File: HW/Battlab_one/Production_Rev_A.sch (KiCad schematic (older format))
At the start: 53 parts, among them IC2 MIC5225-5.0YM5-TR, J1 BANANA_CONN, J3 BANANA_CONN, P1 USB_C_Plug, T1 750315371

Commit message: manf#
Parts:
- AD5248: manf# (none) -> 584-AD5248BRMZ100
- AP2318: manf# (none) -> 621-AP2318M-ADJTRG1
- FTDI232RL1: manf# (none) -> C8690
- IC2: manf# (none) -> C145704
- INA233: manf# (none) -> 595-INA233AIDGST
- ISO1540: manf# (none) -> C179739
- ISO7742: manf# (none) -> 595-ISO7742DBQ
- MSP430: manf# (none) -> C107631
- SN6505: manf# (none) -> C74518
- T1: manf# (none) -> 710-750315371
- USBPROT1: manf# (none) -> 595-TPD2E2U06DRLR
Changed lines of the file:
@@
 	5400 8100 5800 8100
-Wire Wire Line
-	5800 8100 5800 8900
-Wire Wire Line
-	5800 8900 3800 8900
 Wire Wire Line
 	3800 8900 3800 8100
@@
 F 2 "Production_Rev_A:SSOP28DB" H 4900 5100 50  0001 C CNN
 F 3 "" H 4900 5100 50  0001 C CNN
+F 4 "C8690" H 4900 5100 50  0001 C CNN "manf#"
 	1    4900 5100
 	1    0    0    -1
@@
 F 2 "Production_Rev_A:SOIC-8" H 11000 3000 50  0001 C CNN
 F 3 "" H 11000 3000 50  0001 C CNN
+F 4 "621-AP2318M-ADJTRG1" H 11000 3000 50  0001 C CNN "manf#"
 	1    11000 3000
 	1    0    0    -1
@@
 F 2 "Production_Rev_A:VSSOP-10" H 11100 7300 50  0001 C CNN
 F 3 "" H 11100 7300 50  0001 C CNN
+F 4 "595-INA233AIDGST" H 11100 7300 50  0001 C CNN "manf#"
 	1    11100 7300
 	1    0    0    -1
@@
 F 2 "Production_Rev_A:MSOP-10" H 11000 5200 50  0001 C CNN
 F 3 "" H 11000 5200 50  0001 C CNN
+F 4 "584-AD5248BRMZ100" H 11000 5200 50  0001 C CNN "manf#"
 	1    11000 5200
 	1    0    0    -1
@@
 F 2 "Production_Rev_A:PW20" H 5000 2300 50  0001 C CNN
 F 3 "" H 5000 2300 50  0001 C CNN
+F 4 "C107631" H 5000 2300 50  0001 C CNN "manf#"
 	1    5000 2300
 	1    0    0    -1
@@
 F 2 "Production_Rev_A:TOR-6P-HT4_SMT_6PIN_(1201)" H 7900 7400 50  0001 C CNN
 F 3 "" H 7900 7400 50  0001 C CNN
+F 4 "710-750315371" H 7900 7400 50  0001 C CNN "manf#"
 	1    7900 7400
-	1    0    0    -1
-$EndComp
-$Comp
-L Production_Rev_A-eagle-import:SN6505 SN6505
-U 1 1 5779FEE2
-P 5400 8500
-F 0 "SN6505" H 4700 9500 42  0000 L BNN
-F 1 "SN6505" H 4700 8200 42  0000 L BNN
-F 2 "Production_Rev_A:SOT95P280X145-6N" H 5400 8500 50  0001 C CNN
-F 3 "" H 5400 8500 50  0001 C CNN
-	1    5400 8500
 	1    0    0    -1
 $EndComp
@@
 F 2 "Production_Rev_A:SOIC127P600X175-8N" H 9100 5600 50  0001 C CNN
 F 3 "" H 9100 5600 50  0001 C CNN
+F 4 "C179739" H 9100 5600 50  0001 C CNN "manf#"
 	1    9100 5600
 	1    0    0    -1
@@
 F 2 "Production_Rev_A:SOP63P599X175-16N" H 7900 2100 50  0001 C CNN
 F 3 "" H 7900 2100 50  0001 C CNN
+F 4 "595-ISO7742DBQ" H 7900 2100 50  0001 C CNN "manf#"
 	1    7900 2100
 	1    0    0    -1
@@
 F 2 "Production_Rev_A:SOT50P160X60-5N" H 2000 6300 50  0001 C CNN
 F 3 "" H 2000 6300 50  0001 C CNN
+F 4 "595-TPD2E2U06DRLR" H 2000 6300 50  0001 C CNN "manf#"
 	1    2000 6300
 	-1   0    0    1
@@
 F 2 "Production_Rev_A:SOT95P280X130-5N" H 10400 8700 50  0001 C CNN
 F 3 "" H 10400 8700 50  0001 C CNN
+F 4 "C145704" H 10400 8700 50  0001 C CNN "manf#"
 	1    10400 8700
 	1    0    0    -1
@@
 	1505 2165 1650 2165
 Connection ~ 1650 2165
+Wire Wire Line
+	5800 8900 3800 8900
+Wire Wire Line
+	5800 8100 5800 8900
+$Comp
+L Production_Rev_A-eagle-import:SN6505 SN6505
+U 1 1 5779FEE2
+P 5400 8500
+F 0 "SN6505" H 4700 9500 42  0000 L BNN
+F 1 "SN6505" H 4700 8200 42  0000 L BNN
+F 2 "Production_Rev_A:SOT95P280X145-6N" H 5400 8500 50  0001 C CNN
+F 3 "" H 5400 8500 50  0001 C CNN
+F 4 "C74518" H 5400 8500 50  0001 C CNN "manf#"
+	1    5400 8500
+	1    0    0    -1
+$EndComp
 $EndSCHEMATC

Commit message: manf#
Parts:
- C1, C10, C4: manf# (none) -> C123655
- C11, C14, C16, C17, C5, C7, C8: manf# (none) -> C110253
- C12, C13: manf# (none) -> C513774
- C15, C2, C6: manf# (none) -> C141195
- C3: manf# (none) -> C249843
- C9: manf# (none) -> C1845
- D2, D3: manf# (none) -> 863-MBR0520LT1G
- D4: manf# (none) -> C375460
- J1, J3: manf# (none) -> C106273
- P-MOS1: manf# (none) -> C518789
- P1: manf# (none) -> C393939
- R1, R2, R6, R7: manf# (none) -> C104602
- R10, R9: manf# (none) -> C164004
- R11, R12: manf# (none) -> C137353
- R13: manf# (none) -> C702843
- R14, R8: manf# (none) -> C723762
- R15: manf# (none) -> C149672
- R3: manf# (none) -> C104814
- R4, R5: manf# (none) -> C429214
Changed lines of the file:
@@
 F 2 "Production_Rev_A:1206" H 6800 4100 50  0001 C CNN
 F 3 "" H 6800 4100 50  0001 C CNN
+F 4 "C104602" H 6800 4100 50  0001 C CNN "manf#"
 	1    6800 4100
 	0    -1   -1   0
@@
 F 2 "Production_Rev_A:1206" H 7000 4100 50  0001 C CNN
 F 3 "" H 7000 4100 50  0001 C CNN
+F 4 "C104602" H 7000 4100 50  0001 C CNN "manf#"
 	1    7000 4100
 	0    -1   -1   0
@@
 F 2 "Production_Rev_A:1206" H 12300 5400 50  0001 C CNN
 F 3 "" H 12300 5400 50  0001 C CNN
+F 4 "C141195" H 12300 5400 50  0001 C CNN "manf#"
 	1    12300 5400
 	1    0    0    -1
@@
 F 2 "Production_Rev_A:1206" H 14600 3300 50  0001 C CNN
 F 3 "" H 14600 3300 50  0001 C CNN
+F 4 "C149672" H 14600 3300 50  0001 C CNN "manf#"
 	1    14600 3300
 	1    0    0    -1
@@
 F 2 "Production_Rev_A:1206" H 10300 3600 50  0001 C CNN
 F 3 "" H 10300 3600 50  0001 C CNN
+F 4 "C123655" H 10300 3600 50  0001 C CNN "manf#"
 	1    10300 3600
 	-1   0    0    1
@@
 F 2 "Production_Rev_A:PANASONIC_F" H 15700 3000 50  0001 C CNN
 F 3 "" H 15700 3000 50  0001 C CNN
+F 4 "C249843" H 15700 3000 50  0001 C CNN "manf#"
 	1    15700 3000
 	-1   0    0    1
@@
 F 2 "Production_Rev_A:1206" H 4100 3100 50  0001 C CNN
 F 3 "" H 4100 3100 50  0001 C CNN
+F 4 "C110253" H 4100 3100 50  0001 C CNN "manf#"
 	1    4100 3100
 	0    1    1    0
@@
 F 2 "Production_Rev_A:1206" H 4800 1200 50  0001 C CNN
 F 3 "" H 4800 1200 50  0001 C CNN
+F 4 "C429214" H 4800 1200 50  0001 C CNN "manf#"
 	1    4800 1200
 	1    0    0    -1
@@
 F 2 "Production_Rev_A:1206" H 6400 2300 50  0001 C CNN
 F 3 "" H 6400 2300 50  0001 C CNN
+F 4 "C1845" H 6400 2300 50  0001 C CNN "manf#"
 	1    6400 2300
 	0    1    1    0
@@
 F 2 "Production_Rev_A:1206" H 3100 3100 50  0001 C CNN
 F 3 "" H 3100 3100 50  0001 C CNN
+F 4 "C429214" H 3100 3100 50  0001 C CNN "manf#"
 	1    3100 3100
 	-1   0    0    1
@@
 F 2 "Production_Rev_A:1206" H 6500 1400 50  0001 C CNN
 F 3 "" H 6500 1400 50  0001 C CNN
+F 4 "C137353" H 6500 1400 50  0001 C CNN "manf#"
 	1    6500 1400
 	1    0    0    -1
@@
 F 2 "Production_Rev_A:1206" H 16000 3010 50  0001 C CNN
 F 3 "" H 16000 3010 50  0001 C CNN
+F 4 "C110253" H 16000 3010 50  0001 C CNN "manf#"
 	1    16000 3010
 	1    0    0    -1
@@
 F 2 "Production_Rev_A:1206" H 3800 9300 50  0001 C CNN
 F 3 "" H 3800 9300 50  0001 C CNN
+F 4 "C513774" H 3800 9300 50  0001 C CNN "manf#"
 	1    3800 9300
 	1    0    0    -1
@@
 F 2 "Production_Rev_A:SOD3716X117(SOD-123)" H 8800 7100 50  0001 C CNN
 F 3 "" H 8800 7100 50  0001 C CNN
+F 4 "863-MBR0520LT1G" H 8800 7100 50  0001 C CNN "manf#"
 	1    8800 7100
 	1    0    0    -1
@@
 F 2 "Production_Rev_A:SOD3716X117(SOD-123)" H 8900 7700 50  0001 C CNN
 F 3 "" H 8900 7700 50  0001 C CNN
+F 4 "863-MBR0520LT1G" H 8900 7700 50  0001 C CNN "manf#"
 	1    8900 7700
 	1    0    0    -1
@@
 F 2 "Production_Rev_A:1206" H 9300 8100 50  0001 C CNN
 F 3 "" H 9300 8100 50  0001 C CNN
+F 4 "C513774" H 9300 8100 50  0001 C CNN "manf#"
 	1    9300 8100
 	1    0    0    -1
@@
 F 2 "Production_Rev_A:1206" H 9800 8100 50  0001 C CNN
 F 3 "" H 9800 8100 50  0001 C CNN
+F 4 "C110253" H 9800 8100 50  0001 C CNN "manf#"
 	1    9800 8100
 	1    0    0    -1
@@
 F 2 "Production_Rev_A:1206" H 8800 4600 50  0001 C CNN
 F 3 "" H 8800 4600 50  0001 C CNN
+F 4 "C104602" H 8800 4600 50  0001 C CNN "manf#"
 	1    8800 4600
 	0    1    1    0
@@
 F 2 "Production_Rev_A:1206" H 9100 4600 50  0001 C CNN
 F 3 "" H 9100 4600 50  0001 C CNN
+F 4 "C104602" H 9100 4600 50  0001 C CNN "manf#"
 	1    9100 4600
 	0    1    1    0
@@
 F 2 "Production_Rev_A:1206" H 3300 2200 50  0001 C CNN
 F 3 "" H 3300 2200 50  0001 C CNN
+F 4 "C123655" H 3300 2200 50  0001 C CNN "manf#"
 	1    3300 2200
 	-1   0    0    1
@@
 F 2 "Production_Rev_A:1206" H 13900 3300 50  0001 C CNN
 F 3 "" H 13900 3300 50  0001 C CNN
+F 4 "C723762" H 13900 3300 50  0001 C CNN "manf#"
 	1    13900 3300
 	1    0    0    -1
@@
 F 2 "Production_Rev_A:SOT23-3" H 13800 4400 50  0001 C CNN
 F 3 "" H 13800 4400 50  0001 C CNN
+F 4 "C518789" H 13800 4400 50  0001 C CNN "manf#"
 	1    13800 4400
 	0    -1   -1   0
@@
 F 2 "Production_Rev_A:1206" H 6500 1000 50  0001 C CNN
 F 3 "" H 6500 1000 50  0001 C CNN
+F 4 "C137353" H 6500 1000 50  0001 C CNN "manf#"
 	1    6500 1000
 	1    0    0    -1
@@
 F 2 "Production_Rev_A:1206" H 15900 4100 50  0001 C CNN
 F 3 "" H 15900 4100 50  0001 C CNN
+F 4 "C723762" H 15900 4100 50  0001 C CNN "manf#"
 	1    15900 4100
 	-1   0    0    1
@@
 F 2 "Production_Rev_A:1206" H 11600 3600 50  0001 C CNN
 F 3 "" H 11600 3600 50  0001 C CNN
+F 4 "C141195" H 11600 3600 50  0001 C CNN "manf#"
 	1    11600 3600
 	1    0    0    -1
@@
 F 2 "Production_Rev_A:1206" H 7200 1200 50  0001 C CNN
 F 3 "" H 7200 1200 50  0001 C CNN
+F 4 "C110253" H 7200 1200 50  0001 C CNN "manf#"
 	1    7200 1200
 	0    1    1    0
@@
 F 2 "Production_Rev_A:1206" H 8500 1200 50  0001 C CNN
 F 3 "" H 8500 1200 50  0001 C CNN
+F 4 "C110253" H 8500 1200 50  0001 C CNN "manf#"
 	1    8500 1200
 	0    1    1    0
@@
 F 2 "Production_Rev_A:LED-1206" H 13300 1600 50  0001 C CNN
 F 3 "" H 13300 1600 50  0001 C CNN
+F 4 "C375460" H 13300 1600 50  0001 C CNN "manf#"
 	1    13300 1600
 	0    -1   -1   0
@@
 F 2 "Production_Rev_A:1206" H 14100 1900 50  0001 C CNN
 F 3 "" H 14100 1900 50  0001 C CNN
+F 4 "C104814" H 14100 1900 50  0001 C CNN "manf#"
 	1    14100 1900
 	0    -1   -1   0
@@
 F 2 "Production_Rev_A:1206" H 10000 9150 50  0001 C CNN
 F 3 "" H 10000 9150 50  0001 C CNN
+F 4 "C123655" H 10000 9150 50  0001 C CNN "manf#"
 	1    10000 9150
 	1    0    0    -1
@@
 F 2 "Production_Rev_A:1206" H 11800 9290 50  0001 C CNN
 F 3 "" H 11800 9290 50  0001 C CNN
+F 4 "C141195" H 11800 9290 50  0001 C CNN "manf#"
 	1    11800 9290
 	1    0    0    -1
@@
 F 2 "Production_Rev_A:1206" H 7500 3900 50  0001 C CNN
 F 3 "" H 7500 3900 50  0001 C CNN
+F 4 "C110253" H 7500 3900 50  0001 C CNN "manf#"
 	1    7500 3900
 	1    0    0    -1
@@
 F 2 "Production_Rev_A:1206" H 8300 3900 50  0001 C CNN
 F 3 "" H 8300 3900 50  0001 C CNN
+F 4 "C110253" H 8300 3900 50  0001 C CNN "manf#"
 	1    8300 3900
 	1    0    0    -1
@@
 F 2 "Production_Rev_A:BANANA_CONN" H 16700 3300 50  0001 C CNN
 F 3 "" H 16700 3300 50  0001 C CNN
+F 4 "C106273" H 16700 3300 50  0001 C CNN "manf#"
 	1    16700 3300
 	1    0    0    -1
@@
 F 2 "Production_Rev_A:BANANA_CONN" H 16700 2700 50  0001 C CNN
 F 3 "" H 16700 2700 50  0001 C CNN
+F 4 "C106273" H 16700 2700 50  0001 C CNN "manf#"
 	1    16700 2700
 	1    0    0    -1
@@
 F 2 "Production_Rev_A:1206" H 15100 3000 50  0001 C CNN
 F 3 "" H 15100 3000 50  0001 C CNN
+F 4 "C702843" H 15100 3000 50  0001 C CNN "manf#"
 	1    15100 3000
 	0    -1   -1   0
@@
 F 2 "Production_Rev_A:C393939" H 825 2465 50  0001 C CNN
 F 3 "https://www.usb.org/sites/default/files/documents/usb_type-c.zip" H 825 2465 50  0001 C CNN
+F 4 "C393939" H 675 2465 50  0001 C CNN "manf#"
 	1    675  2465
 	1    0    0    -1
@@
 F 2 "Resistor_SMD:R_0805_2012Metric" H 1415 2065 50  0001 C CNN
 F 3 "~" H 1415 2065 50  0001 C CNN
+F 4 "C164004" H 1415 2065 50  0001 C CNN "manf#"
 	1    1415 2065
 	0    1    1    0
@@
 F 2 "Resistor_SMD:R_0805_2012Metric" H 1405 2165 50  0001 C CNN
 F 3 "~" H 1405 2165 50  0001 C CNN
+F 4 "C164004" H 1405 2165 50  0001 C CNN "manf#"
 	1    1405 2165
 	0    -1   -1   0

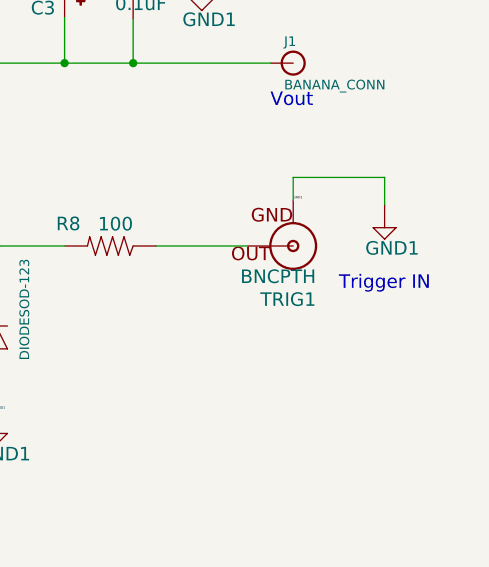
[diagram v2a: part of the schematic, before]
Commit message: Added component
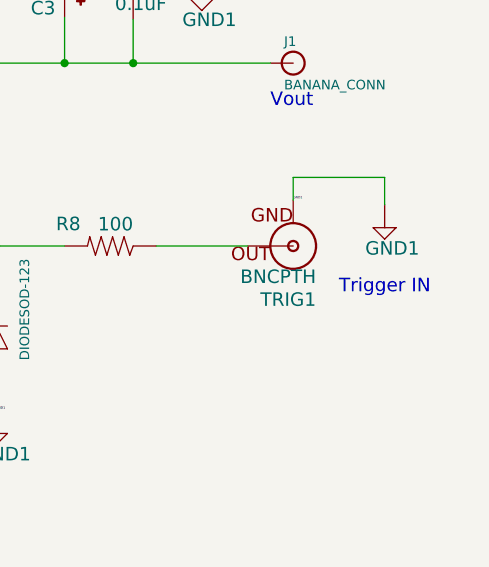
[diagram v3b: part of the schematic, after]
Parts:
- AD5248, AP2318, D2, D3, INA233, ISO7742, T1, USBPROT1: Provedor  (none) -> Mouser
- C1, C10, C11, C12, C13, C14, C15, C16, C17, C2, C3, C4, C5, C6, C7, C8, C9, D4, FTDI232RL1, IC2, ISO1540, J1, J3, MSP430, P-MOS1, P1, R1, R10, R11, R12, R13, R14, R15, R2, R3, R4, R5, R6, R7, R8, R9, SN6505: Provedor  (none) -> LCSC
- D1: Provedor  (none) -> Mouser; manf# (none) -> 512-MBR0530
- JP1: Provedor  (none) -> LCSC; manf# (none) -> C50981
- TRIG1: Provedor  (none) -> Mouser; manf# (none) -> 530-CPBNCPC-010
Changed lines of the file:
@@
 F 3 "" H 4900 5100 50  0001 C CNN
 F 4 "C8690" H 4900 5100 50  0001 C CNN "manf#"
+F 5 "LCSC" H 4900 5100 50  0001 C CNN "Provedor "
 	1    4900 5100
 	1    0    0    -1
@@
 F 3 "" H 6800 4100 50  0001 C CNN
 F 4 "C104602" H 6800 4100 50  0001 C CNN "manf#"
+F 5 "LCSC" H 6800 4100 50  0001 C CNN "Provedor "
 	1    6800 4100
 	0    -1   -1   0
@@
 F 3 "" H 7000 4100 50  0001 C CNN
 F 4 "C104602" H 7000 4100 50  0001 C CNN "manf#"
+F 5 "LCSC" H 7000 4100 50  0001 C CNN "Provedor "
 	1    7000 4100
 	0    -1   -1   0
@@
 F 3 "" H 12300 5400 50  0001 C CNN
 F 4 "C141195" H 12300 5400 50  0001 C CNN "manf#"
+F 5 "LCSC" H 12300 5400 50  0001 C CNN "Provedor "
 	1    12300 5400
 	1    0    0    -1
@@
 F 3 "" H 14600 3300 50  0001 C CNN
 F 4 "C149672" H 14600 3300 50  0001 C CNN "manf#"
+F 5 "LCSC" H 14600 3300 50  0001 C CNN "Provedor "
 	1    14600 3300
 	1    0    0    -1
@@
 F 3 "" H 11000 3000 50  0001 C CNN
 F 4 "621-AP2318M-ADJTRG1" H 11000 3000 50  0001 C CNN "manf#"
+F 5 "Mouser" H 11000 3000 50  0001 C CNN "Provedor "
 	1    11000 3000
 	1    0    0    -1
@@
 F 3 "" H 11100 7300 50  0001 C CNN
 F 4 "595-INA233AIDGST" H 11100 7300 50  0001 C CNN "manf#"
+F 5 "Mouser" H 11100 7300 50  0001 C CNN "Provedor "
 	1    11100 7300
 	1    0    0    -1
@@
 F 3 "" H 11000 5200 50  0001 C CNN
 F 4 "584-AD5248BRMZ100" H 11000 5200 50  0001 C CNN "manf#"
+F 5 "Mouser" H 11000 5200 50  0001 C CNN "Provedor "
 	1    11000 5200
 	1    0    0    -1
@@
 F 3 "" H 10300 3600 50  0001 C CNN
 F 4 "C123655" H 10300 3600 50  0001 C CNN "manf#"
+F 5 "LCSC" H 10300 3600 50  0001 C CNN "Provedor "
 	1    10300 3600
 	-1   0    0    1
@@
 F 3 "" H 15700 3000 50  0001 C CNN
 F 4 "C249843" H 15700 3000 50  0001 C CNN "manf#"
+F 5 "LCSC" H 15700 3000 50  0001 C CNN "Provedor "
 	1    15700 3000
 	-1   0    0    1
@@
 F 3 "" H 4100 3100 50  0001 C CNN
 F 4 "C110253" H 4100 3100 50  0001 C CNN "manf#"
+F 5 "LCSC" H 4100 3100 50  0001 C CNN "Provedor "
 	1    4100 3100
 	0    1    1    0
@@
 F 3 "" H 4800 1200 50  0001 C CNN
 F 4 "C429214" H 4800 1200 50  0001 C CNN "manf#"
+F 5 "LCSC" H 4800 1200 50  0001 C CNN "Provedor "
 	1    4800 1200
 	1    0    0    -1
@@
 F 3 "" H 6400 2300 50  0001 C CNN
 F 4 "C1845" H 6400 2300 50  0001 C CNN "manf#"
+F 5 "LCSC" H 6400 2300 50  0001 C CNN "Provedor "
 	1    6400 2300
 	0    1    1    0
@@
 F 3 "" H 3100 3100 50  0001 C CNN
 F 4 "C429214" H 3100 3100 50  0001 C CNN "manf#"
+F 5 "LCSC" H 3100 3100 50  0001 C CNN "Provedor "
 	1    3100 3100
 	-1   0    0    1
@@
 F 3 "" H 5000 2300 50  0001 C CNN
 F 4 "C107631" H 5000 2300 50  0001 C CNN "manf#"
+F 5 "LCSC" H 5000 2300 50  0001 C CNN "Provedor "
 	1    5000 2300
 	1    0    0    -1
@@
 F 3 "" H 6500 1400 50  0001 C CNN
 F 4 "C137353" H 6500 1400 50  0001 C CNN "manf#"
+F 5 "LCSC" H 6500 1400 50  0001 C CNN "Provedor "
 	1    6500 1400
 	1    0    0    -1
@@
 F 3 "" H 16000 3010 50  0001 C CNN
 F 4 "C110253" H 16000 3010 50  0001 C CNN "manf#"
+F 5 "LCSC" H 16000 3010 50  0001 C CNN "Provedor "
 	1    16000 3010
 	1    0    0    -1
@@
 F 2 "Production_Rev_A:1X06" H 7100 6300 50  0001 C CNN
 F 3 "" H 7100 6300 50  0001 C CNN
+F 4 "LCSC" H 7100 6300 50  0001 C CNN "Provedor "
+F 5 "C50981" H 7100 6300 50  0001 C CNN "manf#"
 	1    7100 6300
 	-1   0    0    1
@@
 F 3 "" H 7900 7400 50  0001 C CNN
 F 4 "710-750315371" H 7900 7400 50  0001 C CNN "manf#"
+F 5 "Mouser" H 7900 7400 50  0001 C CNN "Provedor "
 	1    7900 7400
 	1    0    0    -1
@@
 F 3 "" H 9100 5600 50  0001 C CNN
 F 4 "C179739" H 9100 5600 50  0001 C CNN "manf#"
+F 5 "LCSC" H 9100 5600 50  0001 C CNN "Provedor "
 	1    9100 5600
 	1    0    0    -1
@@
 F 3 "" H 3800 9300 50  0001 C CNN
 F 4 "C513774" H 3800 9300 50  0001 C CNN "manf#"
+F 5 "LCSC" H 3800 9300 50  0001 C CNN "Provedor "
 	1    3800 9300
 	1    0    0    -1
@@
 F 3 "" H 8800 7100 50  0001 C CNN
 F 4 "863-MBR0520LT1G" H 8800 7100 50  0001 C CNN "manf#"
+F 5 "Mouser" H 8800 7100 50  0001 C CNN "Provedor "
 	1    8800 7100
 	1    0    0    -1
@@
 F 3 "" H 8900 7700 50  0001 C CNN
 F 4 "863-MBR0520LT1G" H 8900 7700 50  0001 C CNN "manf#"
+F 5 "Mouser" H 8900 7700 50  0001 C CNN "Provedor "
 	1    8900 7700
 	1    0    0    -1
@@
 F 3 "" H 9300 8100 50  0001 C CNN
 F 4 "C513774" H 9300 8100 50  0001 C CNN "manf#"
+F 5 "LCSC" H 9300 8100 50  0001 C CNN "Provedor "
 	1    9300 8100
 	1    0    0    -1
@@
 F 3 "" H 9800 8100 50  0001 C CNN
 F 4 "C110253" H 9800 8100 50  0001 C CNN "manf#"
+F 5 "LCSC" H 9800 8100 50  0001 C CNN "Provedor "
 	1    9800 8100
 	1    0    0    -1
@@
 F 3 "" H 8800 4600 50  0001 C CNN
 F 4 "C104602" H 8800 4600 50  0001 C CNN "manf#"
+F 5 "LCSC" H 8800 4600 50  0001 C CNN "Provedor "
 	1    8800 4600
 	0    1    1    0
@@
 F 3 "" H 9100 4600 50  0001 C CNN
 F 4 "C104602" H 9100 4600 50  0001 C CNN "manf#"
+F 5 "LCSC" H 9100 4600 50  0001 C CNN "Provedor "
 	1    9100 4600
 	0    1    1    0
@@
 F 3 "" H 3300 2200 50  0001 C CNN
 F 4 "C123655" H 3300 2200 50  0001 C CNN "manf#"
+F 5 "LCSC" H 3300 2200 50  0001 C CNN "Provedor "
 	1    3300 2200
 	-1   0    0    1
@@
 F 3 "" H 13900 3300 50  0001 C CNN
 F 4 "C723762" H 13900 3300 50  0001 C CNN "manf#"
+F 5 "LCSC" H 13900 3300 50  0001 C CNN "Provedor "
 	1    13900 3300
 	1    0    0    -1
@@
 F 3 "" H 13800 4400 50  0001 C CNN
 F 4 "C518789" H 13800 4400 50  0001 C CNN "manf#"
+F 5 "LCSC" H 13800 4400 50  0001 C CNN "Provedor "
 	1    13800 4400
 	0    -1   -1   0
@@
 F 3 "" H 6500 1000 50  0001 C CNN
 F 4 "C137353" H 6500 1000 50  0001 C CNN "manf#"
+F 5 "LCSC" H 6500 1000 50  0001 C CNN "Provedor "
 	1    6500 1000
 	1    0    0    -1
@@
 F 3 "" H 7900 2100 50  0001 C CNN
 F 4 "595-ISO7742DBQ" H 7900 2100 50  0001 C CNN "manf#"
+F 5 "Mouser" H 7900 2100 50  0001 C CNN "Provedor "
 	1    7900 2100
 	1    0    0    -1
@@
 F 3 "" H 2000 6300 50  0001 C CNN
 F 4 "595-TPD2E2U06DRLR" H 2000 6300 50  0001 C CNN "manf#"
+F 5 "Mouser " H 2000 6300 50  0001 C CNN "Provedor "
 	1    2000 6300
 	-1   0    0    1
@@
 F 3 "" H 15900 4100 50  0001 C CNN
 F 4 "C723762" H 15900 4100 50  0001 C CNN "manf#"
+F 5 "LCSC" H 15900 4100 50  0001 C CNN "Provedor "
 	1    15900 4100
 	-1   0    0    1
@@
 F 3 "" H 11600 3600 50  0001 C CNN
 F 4 "C141195" H 11600 3600 50  0001 C CNN "manf#"
+F 5 "LCSC" H 11600 3600 50  0001 C CNN "Provedor "
 	1    11600 3600
 	1    0    0    -1
@@
 F 3 "" H 7200 1200 50  0001 C CNN
 F 4 "C110253" H 7200 1200 50  0001 C CNN "manf#"
+F 5 "LCSC" H 7200 1200 50  0001 C CNN "Provedor "
 	1    7200 1200
 	0    1    1    0
@@
 F 3 "" H 8500 1200 50  0001 C CNN
 F 4 "C110253" H 8500 1200 50  0001 C CNN "manf#"
+F 5 "LCSC" H 8500 1200 50  0001 C CNN "Provedor "
 	1    8500 1200
 	0    1    1    0
@@
 F 3 "" H 13300 1600 50  0001 C CNN
 F 4 "C375460" H 13300 1600 50  0001 C CNN "manf#"
+F 5 "LCSC" H 13300 1600 50  0001 C CNN "Provedor "
 	1    13300 1600
 	0    -1   -1   0
@@
 F 3 "" H 14100 1900 50  0001 C CNN
 F 4 "C104814" H 14100 1900 50  0001 C CNN "manf#"
+F 5 "LCSC" H 14100 1900 50  0001 C CNN "Provedor "
 	1    14100 1900
 	0    -1   -1   0
@@
 F 3 "" H 10000 9150 50  0001 C CNN
 F 4 "C123655" H 10000 9150 50  0001 C CNN "manf#"
+F 5 "LCSC" H 10000 9150 50  0001 C CNN "Provedor "
 	1    10000 9150
 	1    0    0    -1
@@
 F 3 "" H 11800 9290 50  0001 C CNN
 F 4 "C141195" H 11800 9290 50  0001 C CNN "manf#"
+F 5 "LCSC" H 11800 9290 50  0001 C CNN "Provedor "
 	1    11800 9290
 	1    0    0    -1
@@
 F 3 "" H 10400 8700 50  0001 C CNN
 F 4 "C145704" H 10400 8700 50  0001 C CNN "manf#"
+F 5 "LCSC" H 10400 8700 50  0001 C CNN "Provedor "
 	1    10400 8700
 	1    0    0    -1
@@
 F 3 "" H 7500 3900 50  0001 C CNN
 F 4 "C110253" H 7500 3900 50  0001 C CNN "manf#"
+F 5 "LCSC" H 7500 3900 50  0001 C CNN "Provedor "
 	1    7500 3900
 	1    0    0    -1
@@
 F 3 "" H 8300 3900 50  0001 C CNN
 F 4 "C110253" H 8300 3900 50  0001 C CNN "manf#"
+F 5 "LCSC" H 8300 3900 50  0001 C CNN "Provedor "
 	1    8300 3900
 	1    0    0    -1
@@
 F 2 "Production_Rev_A:BNC" H 16700 4100 50  0001 C CNN
 F 3 "" H 16700 4100 50  0001 C CNN
+F 4 "Mouser" H 16700 4100 50  0001 C CNN "Provedor "
+F 5 "530-CPBNCPC-010" H 16700 4100 50  0001 C CNN "manf#"
 	1    16700 4100
 	-1   0    0    1
@@
 F 3 "" H 16700 3300 50  0001 C CNN
 F 4 "C106273" H 16700 3300 50  0001 C CNN "manf#"
+F 5 "LCSC" H 16700 3300 50  0001 C CNN "Provedor "
 	1    16700 3300
 	1    0    0    -1
@@
 F 3 "" H 16700 2700 50  0001 C CNN
 F 4 "C106273" H 16700 2700 50  0001 C CNN "manf#"
+F 5 "LCSC" H 16700 2700 50  0001 C CNN "Provedor "
 	1    16700 2700
 	1    0    0    -1
@@
 F 2 "Production_Rev_A:SOD-123" H 15400 4500 50  0001 C CNN
 F 3 "" H 15400 4500 50  0001 C CNN
+F 4 "Mouser" H 15400 4500 50  0001 C CNN "Provedor "
+F 5 "512-MBR0530" H 15400 4500 50  0001 C CNN "manf#"
 	1    15400 4500
 	0    -1   -1   0
@@
 F 3 "" H 15100 3000 50  0001 C CNN
 F 4 "C702843" H 15100 3000 50  0001 C CNN "manf#"
+F 5 "LCSC" H 15100 3000 50  0001 C CNN "Provedor "
 	1    15100 3000
 	0    -1   -1   0
@@
 Text Notes 16600 3500 0    59   ~ 0
 Vout
-Text Notes 16900 4300 0    59   ~ 0
+Text Notes 16900 4315 0    59   ~ 0
 Trigger IN
 Text Notes 7370 6510 0    59   ~ 0
@@
 F 3 "https://www.usb.org/sites/default/files/documents/usb_type-c.zip" H 825 2465 50  0001 C CNN
 F 4 "C393939" H 675 2465 50  0001 C CNN "manf#"
+F 5 "LCSC" H 675 2465 50  0001 C CNN "Provedor "
 	1    675  2465
 	1    0    0    -1
@@
 F 3 "~" H 1415 2065 50  0001 C CNN
 F 4 "C164004" H 1415 2065 50  0001 C CNN "manf#"
+F 5 "LCSC" H 1415 2065 50  0001 C CNN "Provedor "
 	1    1415 2065
 	0    1    1    0
@@
 F 3 "~" H 1405 2165 50  0001 C CNN
 F 4 "C164004" H 1405 2165 50  0001 C CNN "manf#"
+F 5 "LCSC" H 1405 2165 50  0001 C CNN "Provedor "
 	1    1405 2165
 	0    -1   -1   0
@@
 F 3 "" H 5400 8500 50  0001 C CNN
 F 4 "C74518" H 5400 8500 50  0001 C CNN "manf#"
+F 5 "LCSC" H 5400 8500 50  0001 C CNN "Provedor "
 	1    5400 8500
 	1    0    0    -1
